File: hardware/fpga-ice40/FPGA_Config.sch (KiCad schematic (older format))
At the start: 5 parts, among them U1 iCE40HX4K-TQ144, U10 MC74HC1G08DTT1G, X1 50MHz

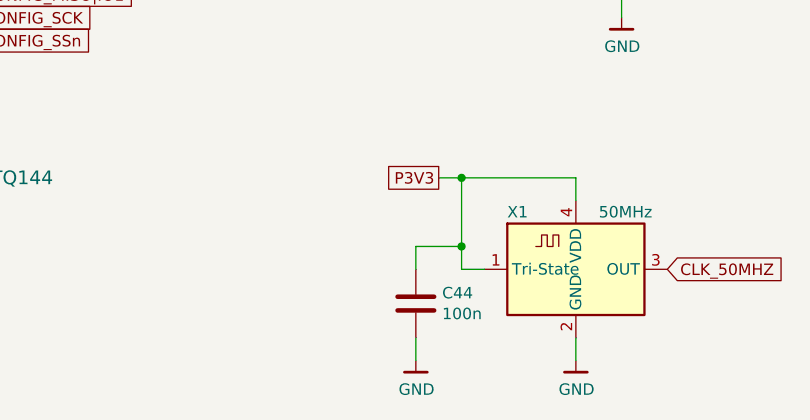
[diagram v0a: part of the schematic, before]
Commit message: Completed verification of all pins for all symbols
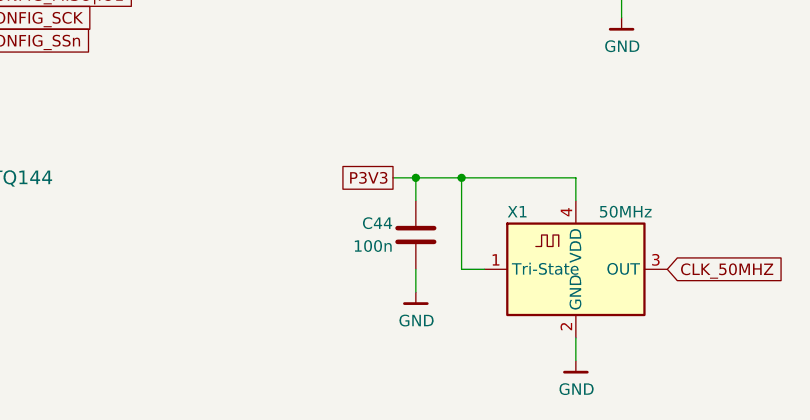
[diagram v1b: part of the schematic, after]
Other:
- moved on the sheet: C44
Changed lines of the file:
@@
 F 1 "50MHz" H 6850 5300 50  0000 L CNN
 F 2 "ng_time:Oscillator_2.5x2.0" H 7200 4700 50  0001 C CNN
-F 3 "https://www.ecsxtal.com/store/pdf/ECS-2520MV.pdf" H 6575 5175 50  0001 C CNN
+F 3 "https://ecsxtal.com/store/pdf/ECS-2520MV.pdf" H 6575 5175 50  0001 C CNN
 F 4 "ECS-2520MV-500-BN-TR" H 6750 5050 50  0001 C CNN "MPN"
 	1    6750 5050
@@
 	1    0    0    -1
 $EndComp
-Text GLabel 6150 4650 0    50   UnSpc ~ 0
+Text GLabel 5950 4650 0    50   UnSpc ~ 0
 P3V3
 Wire Wire Line
 	6350 5050 6250 5050
 Wire Wire Line
-	6250 5050 6250 4950
-Wire Wire Line
 	6250 4650 6750 4650
 Wire Wire Line
 	6750 4650 6750 4750
-Wire Wire Line
-	6150 4650 6250 4650
 Wire Wire Line
 	6750 5450 6750 5350
@@
 CLK_50MHZ
 $Comp
-L Device:C C?
-U 1 1 5F5C1BD0
-P 6050 5200
-AR Path="/5F5C1BD0" Ref="C?"  Part="1"
-AR Path="/5F5B53E5/5F5C1BD0" Ref="C44"  Part="1"
-F 0 "C44" H 6165 5246 50  0000 L CNN
-F 1 "100n" H 6165 5155 50  0000 L CNN
-F 2 "Capacitor_SMD:C_0603_1608Metric" H 6088 5050 50  0001 C CNN
-F 3 "~" H 6050 5200 50  0001 C CNN
-F 4 "CL10B104KB8NNNC" H 6050 5200 50  0001 C CNN "MPN"
-	1    6050 5200
-	1    0    0    -1
-$EndComp
-$Comp
 L ng_power:GND #PWR?
 U 1 1 5F5C1BD6
-P 6050 5450
+P 6050 5150
 AR Path="/5F5C1BD6" Ref="#PWR?"  Part="1"
 AR Path="/5F5B53E5/5F5C1BD6" Ref="#PWR031"  Part="1"
-F 0 "#PWR031" H 6050 5200 50  0001 C CNN
-F 1 "GND" H 6053 5324 50  0000 C CNN
-F 2 "" H 5950 5100 50  0001 C CNN
-F 3 "" H 6050 5450 50  0001 C CNN
-	1    6050 5450
-	1    0    0    -1
-$EndComp
-Wire Wire Line
-	6050 5450 6050 5350
-Wire Wire Line
-	6050 5050 6050 4950
-Wire Wire Line
-	6050 4950 6250 4950
-Connection ~ 6250 4950
-Wire Wire Line
-	6250 4950 6250 4650
+F 0 "#PWR031" H 6050 4900 50  0001 C CNN
+F 1 "GND" H 6053 5024 50  0000 C CNN
+F 2 "" H 5950 4800 50  0001 C CNN
+F 3 "" H 6050 5150 50  0001 C CNN
+	1    6050 5150
+	1    0    0    -1
+$EndComp
+Wire Wire Line
+	6050 5150 6050 5050
 Connection ~ 6250 4650
 $Comp
@@
 F 1 "MC74HC1G08DTT1G" H 7000 3900 50  0000 L CNN
 F 2 "Package_TO_SOT_SMD:SOT-23-5" H 6950 3750 50  0001 C CNN
-F 3 "http://www.ti.com/lit/sg/scyt129e/scyt129e.pdf" H 6950 3750 50  0001 C CNN
+F 3 "https://www.onsemi.com/pub/Collateral/MC74HC1G08-D.PDF" H 6950 3750 50  0001 C CNN
 F 4 "MC74HC1G08DTT1G" H 6950 3750 50  0001 C CNN "MPN"
 	1    6950 3750
@@
 Wire Wire Line
 	6450 2900 6550 2900
+Wire Wire Line
+	6250 4650 6250 5050
+Wire Wire Line
+	5950 4650 6050 4650
+Wire Wire Line
+	6050 4750 6050 4650
+Connection ~ 6050 4650
+Wire Wire Line
+	6050 4650 6250 4650
+$Comp
+L Device:C C?
+U 1 1 5F5C1BD0
+P 6050 4900
+AR Path="/5F5C1BD0" Ref="C?"  Part="1"
+AR Path="/5F5B53E5/5F5C1BD0" Ref="C44"  Part="1"
+F 0 "C44" H 5950 4950 50  0000 R CNN
+F 1 "100n" H 5950 4850 50  0000 R CNN
+F 2 "Capacitor_SMD:C_0603_1608Metric" H 6088 4750 50  0001 C CNN
+F 3 "~" H 6050 4900 50  0001 C CNN
+F 4 "CL10B104KB8NNNC" H 6050 4900 50  0001 C CNN "MPN"
+	1    6050 4900
+	1    0    0    -1
+$EndComp
 $EndSCHEMATC
